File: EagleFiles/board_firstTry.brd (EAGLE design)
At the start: 48 parts

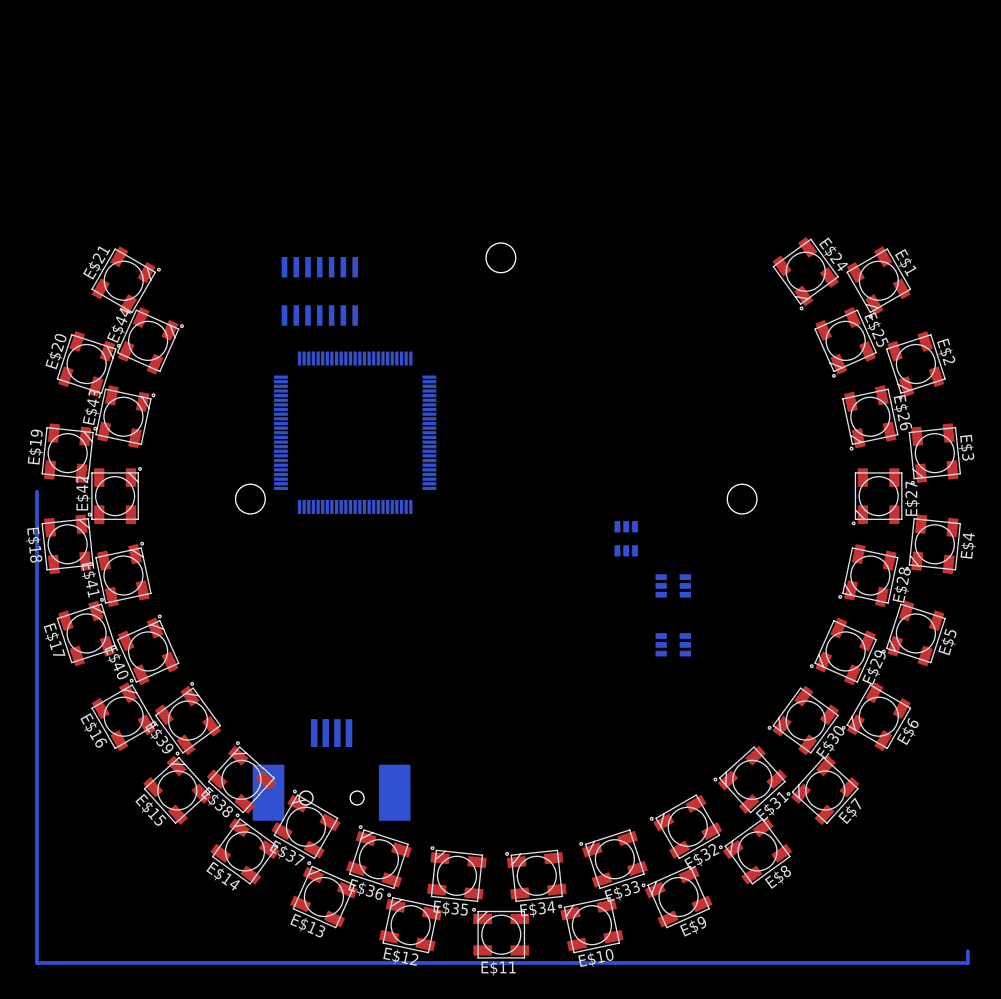
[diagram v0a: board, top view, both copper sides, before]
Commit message: updated eagle
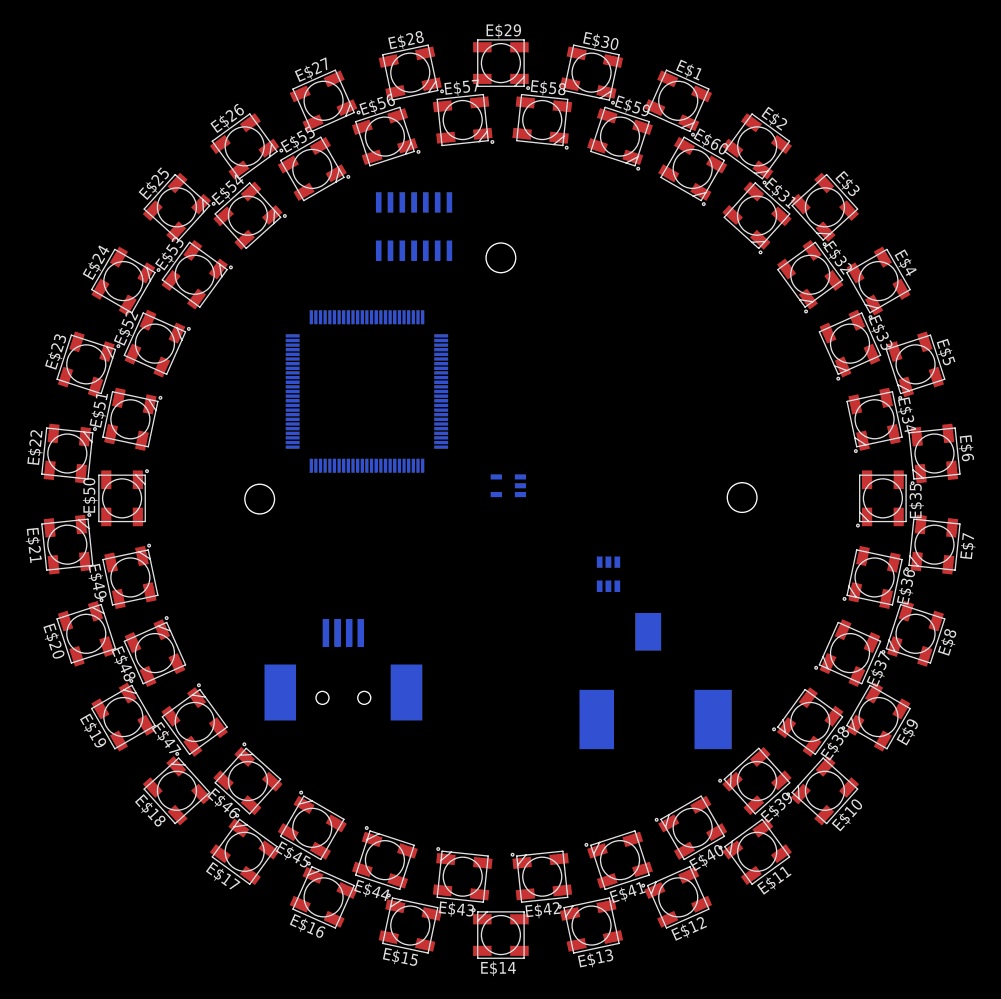
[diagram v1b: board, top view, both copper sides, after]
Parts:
- added 74HCT: (no value), analog-devices:SO14
- added E$49, E$50, E$51, E$52, E$53, E$54, E$55, E$56, E$57, E$58, E$59, E$60: (no value), WS2812B:WS2812B
- added LDO: (no value), analog-devices:SOT23-5
- added LTC4412: (no value), linear-technology:TSOT23-6
- added PWR: (no value), RASM7X2:RASM7X2
- added STM32F7: (no value), STM32F407Vx_LQFP100:LQFP100
- added USB-B: (no value), usb:USB-B-SMT
- E$22: device STM32F407Vx_LQFP100:LQFP100 -> WS2812B:WS2812B
- E$23: device div:USB-B-SMD -> WS2812B:WS2812B
- E$45: device analog-devices:SO14 -> WS2812B:WS2812B
- E$46, E$47, E$48: device linear-technology:TSOT23-6 -> WS2812B:WS2812B
- moved E$24 73.6 mm to (9.31, 73.5), turned to 60 degrees
- moved E$30 73.5 mm to (59.8, 96.0), turned to 348 degrees
- moved E$25 73.5 mm to (15.1, 81.4), turned to 48 degrees
- moved E$29 73.5 mm to (50.0, 97.0), turned to 0 degrees
- moved E$26 73.5 mm to (22.4, 88.0), turned to 36 degrees
- moved E$28 73.5 mm to (40.2, 96.0), turned to 12 degrees
- moved E$27 73.4 mm to (30.9, 92.9), turned to 24 degrees
- moved E$40 61.7 mm to (70.7, 14.6), turned to 210 degrees
- moved E$41 61.7 mm to (62.8, 11.1), turned to 198 degrees
- moved E$39 61.7 mm to (77.6, 19.6), turned to 222 degrees
- moved E$42 61.7 mm to (54.5, 9.30), turned to 186 degrees
- moved E$38 61.6 mm to (83.3, 26.0), turned to 234 degrees
- moved E$43 61.6 mm to (45.9, 9.30), turned to 174 degrees
- moved E$37 61.5 mm to (87.6, 33.4), turned to 246 degrees
- moved E$44 61.5 mm to (37.5, 11.1), turned to 162 degrees
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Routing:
- net S$1: track 152.4 -> 0.00 mm
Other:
- board text added: "Mosfets"
- board text added: "USB-Datenleitung"
